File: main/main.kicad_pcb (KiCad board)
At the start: 2 copper layers, 22 parts, among them J1 VCC12V, J2 GND, J3 RX, J4 TX, J5 VCC5V, J6 OUTGND, J7 RX3V, J8 TX3V, Q1 BSS138, Q2 BSS138, U1 L7805ABV-DG, U2 LD1117S33TR_SOT223

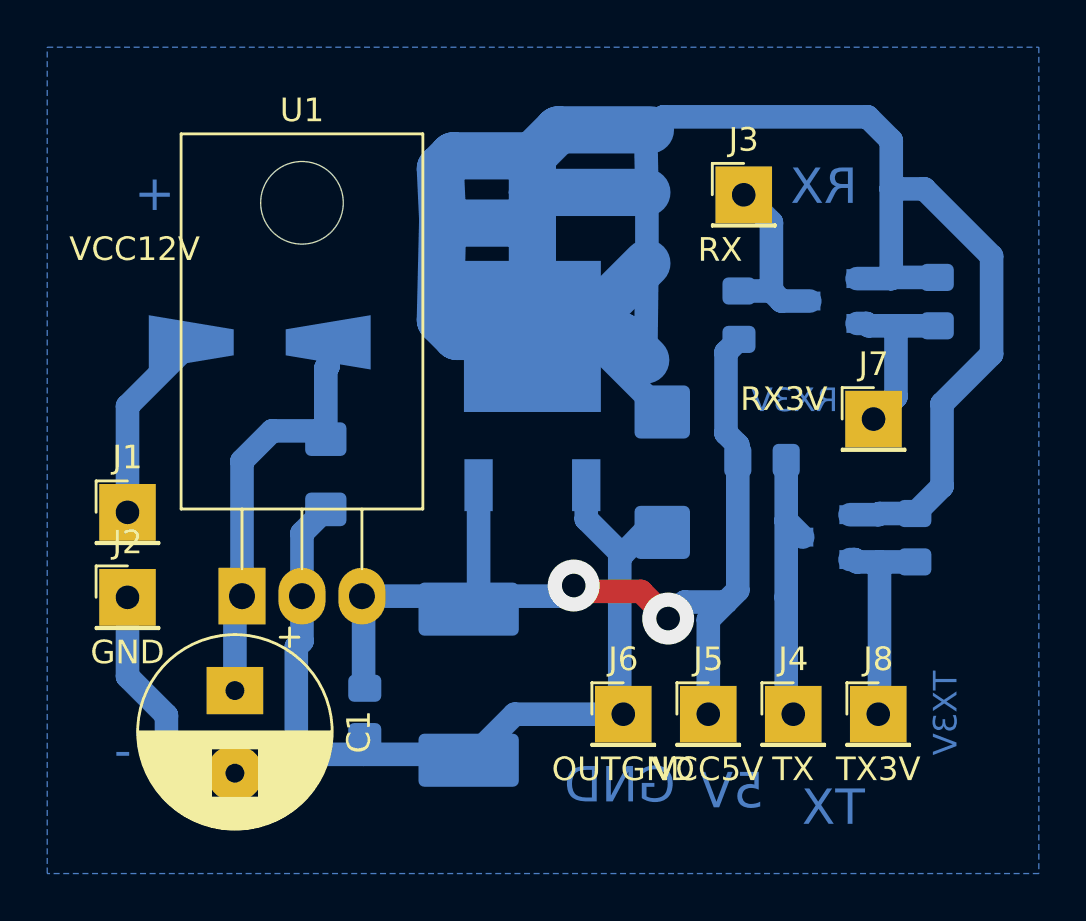
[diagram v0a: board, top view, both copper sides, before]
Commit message: update
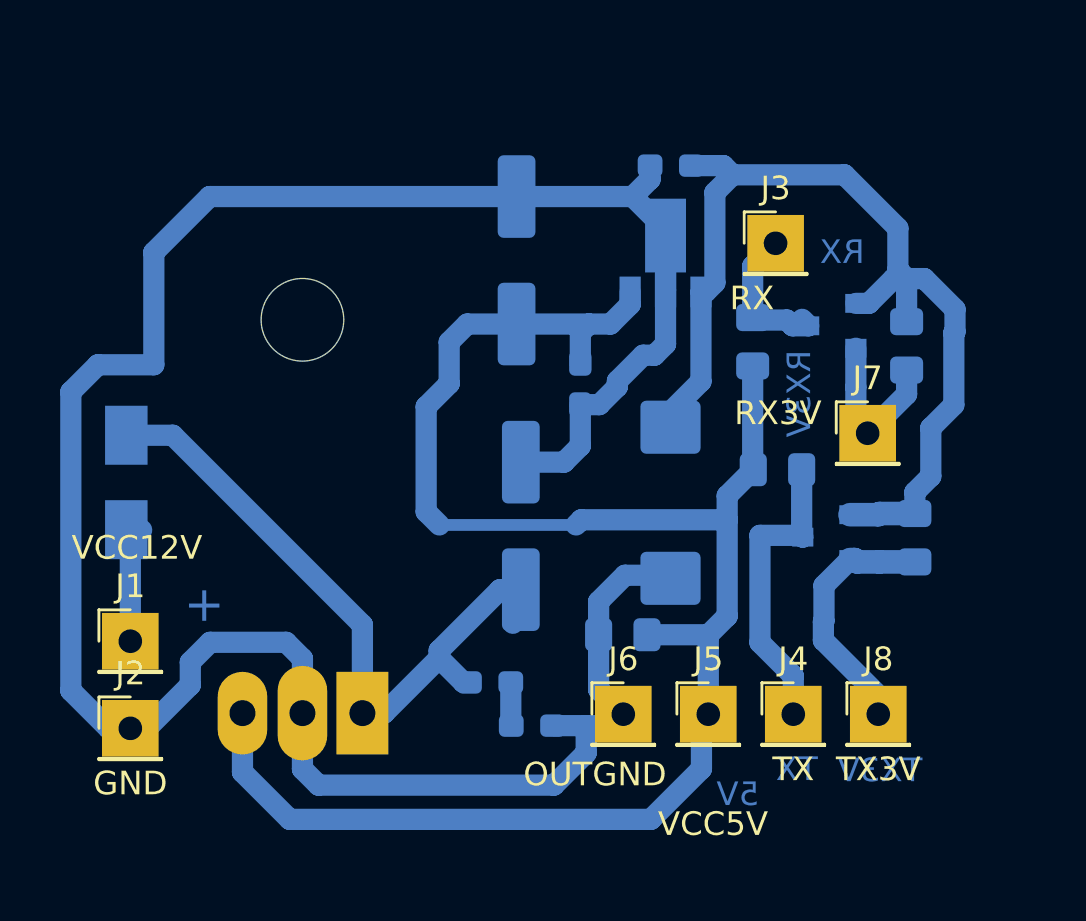
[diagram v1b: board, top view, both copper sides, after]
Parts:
- removed U2: LD1117S33TR_SOT223, Package_TO_SOT_SMD:TO-252-2
- added C6: CP, Capacitor_SMD:CP_Elec_6.3x3, B.Cu at (112.9, 121.0)
- added C7: 47uF, Capacitor_SMD:C_0805_2012Metric_Pad1.15x1.40mm_HandSolder, B.Cu at (117.4, 136.9)
- added C8: CP, Capacitor_Tantalum_SMD:CP_EIA-7343-30_AVX-N_Pad2.25x2.55mm_HandSolder, B.Cu at (119.4, 131.3)
- added U3: L78L33_SOT89, Package_TO_SOT_SMD:SOT-89-3, B.Cu at (119.2, 120.7)
- C1: value 0.33uF -> 1uF; footprint Capacitor_THT:CP_Radial_D8.0mm_P3.50mm -> Capacitor_SMD:C_0603_1608Metric_Pad1.05x0.95mm_HandSolder; moved to B.Cu
- C2: value 0.1uF -> 1uF; footprint Capacitor_SMD:C_0805_2012Metric_Pad1.15x1.40mm_HandSolder -> Capacitor_SMD:C_0603_1608Metric_Pad1.05x0.95mm_HandSolder
- C3: value 100uF -> CP; footprint Capacitor_Tantalum_SMD:CP_EIA-7360-38_Kemet-E_Pad2.25x4.25mm_HandSolder -> Capacitor_SMD:CP_Elec_6.3x3
- C4: value 100uF -> 0.1uF; footprint Capacitor_Tantalum_SMD:CP_EIA-6032-28_Kemet-C_Pad2.25x2.35mm_HandSolder -> Capacitor_SMD:C_0603_1608Metric_Pad1.05x0.95mm_HandSolder
- C5: footprint Capacitor_SMD:C_1206_3216Metric_Pad1.42x1.75mm_HandSolder -> Capacitor_SMD:C_0603_1608Metric_Pad1.05x0.95mm_HandSolder
- D1: footprint Diode_SMD:D_SMA-SMB_Universal_Handsoldering -> Diode_SMD:D_SMA
- U1: value L7805ABV-DG -> KIA7805API; moved to B.Cu
- moved C4 13.0 mm to (119.4, 117.0), turned to 180 degrees
- moved C5 11.4 mm to (115.6, 126.3)
- moved C1 10.8 mm to (111.8, 138.9), turned to 0 degrees
- moved D1 8.19 mm to (96.3, 130.4), turned to 270 degrees
- moved U1 7.11 mm to (106.3, 140.2), turned to 180 degrees
- moved C2 7.10 mm to (113.5, 140.7), turned to 0 degrees
- moved C3 7.08 mm to (113.1, 132.3), turned to 90 degrees
- moved J2 5.55 mm to (96.5, 140.8)
- moved J1 5.46 mm to (96.5, 137.2)
- moved J3 2.46 mm to (123.8, 120.3)
- moved R1 2.28 mm to (129.4, 124.7)
- moved R2 1.27 mm to (122.9, 124.5)
- moved Q1 1.05 mm to (126.2, 123.8)
- moved R4 0.76 mm to (123.9, 129.9)
- moved J7 0.65 mm to (127.8, 128.3)
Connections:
- net LV1 renamed LV1RX3V
- net LV2 renamed LV2TX3V
- net Net-(D1-Pad2) renamed /VCC12
- C1 pad 2: /GND -> Net-(C1-Pad2)
- C2 pad 1: 5V -> Net-(C1-Pad2)
- C3 pad 1: 5V -> /VIN
- C5 pad 1: /VIN -> 5V
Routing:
- net 3V3: track 105.1 -> 43.2 mm
- net /GND: track 53.4 -> 104.4 mm
- net 5V: track 41.6 -> 75.6 mm, vias 2 -> 0
- net /VIN: track 18.3 -> 27.9 mm
- net /VCC12: track 8.32 -> 5.47 mm
- net Net-(C1-Pad2): track 0.00 -> 1.84 mm
- net LV2TX3V: track 9.26 -> 10.8 mm
- net HV1: track 7.74 -> 6.45 mm
- net HV2: track 11.9 -> 12.9 mm
- net LV1RX3V: track 7.78 -> 7.17 mm
- removed copper zone on B.Cu, net /GND
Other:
- board text removed: "-"
- board text removed: "GND"
